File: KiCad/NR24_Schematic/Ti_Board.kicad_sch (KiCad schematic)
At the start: 23 parts, among them J5 J1 Pin J3 Pin, J5 J12 (CAN Interface w/ Transce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, J5 J4 Pin J2 Pin, J5 J5 Pin J7 Pin, J5 J8 Pin J6 Pin, J5 XBEE PRO, J6 SpeakON_NL2, Q1 Q_NMOS_DGS, Q2 Q_NMOS_DGS, Q3 Q_NMOS_DGS

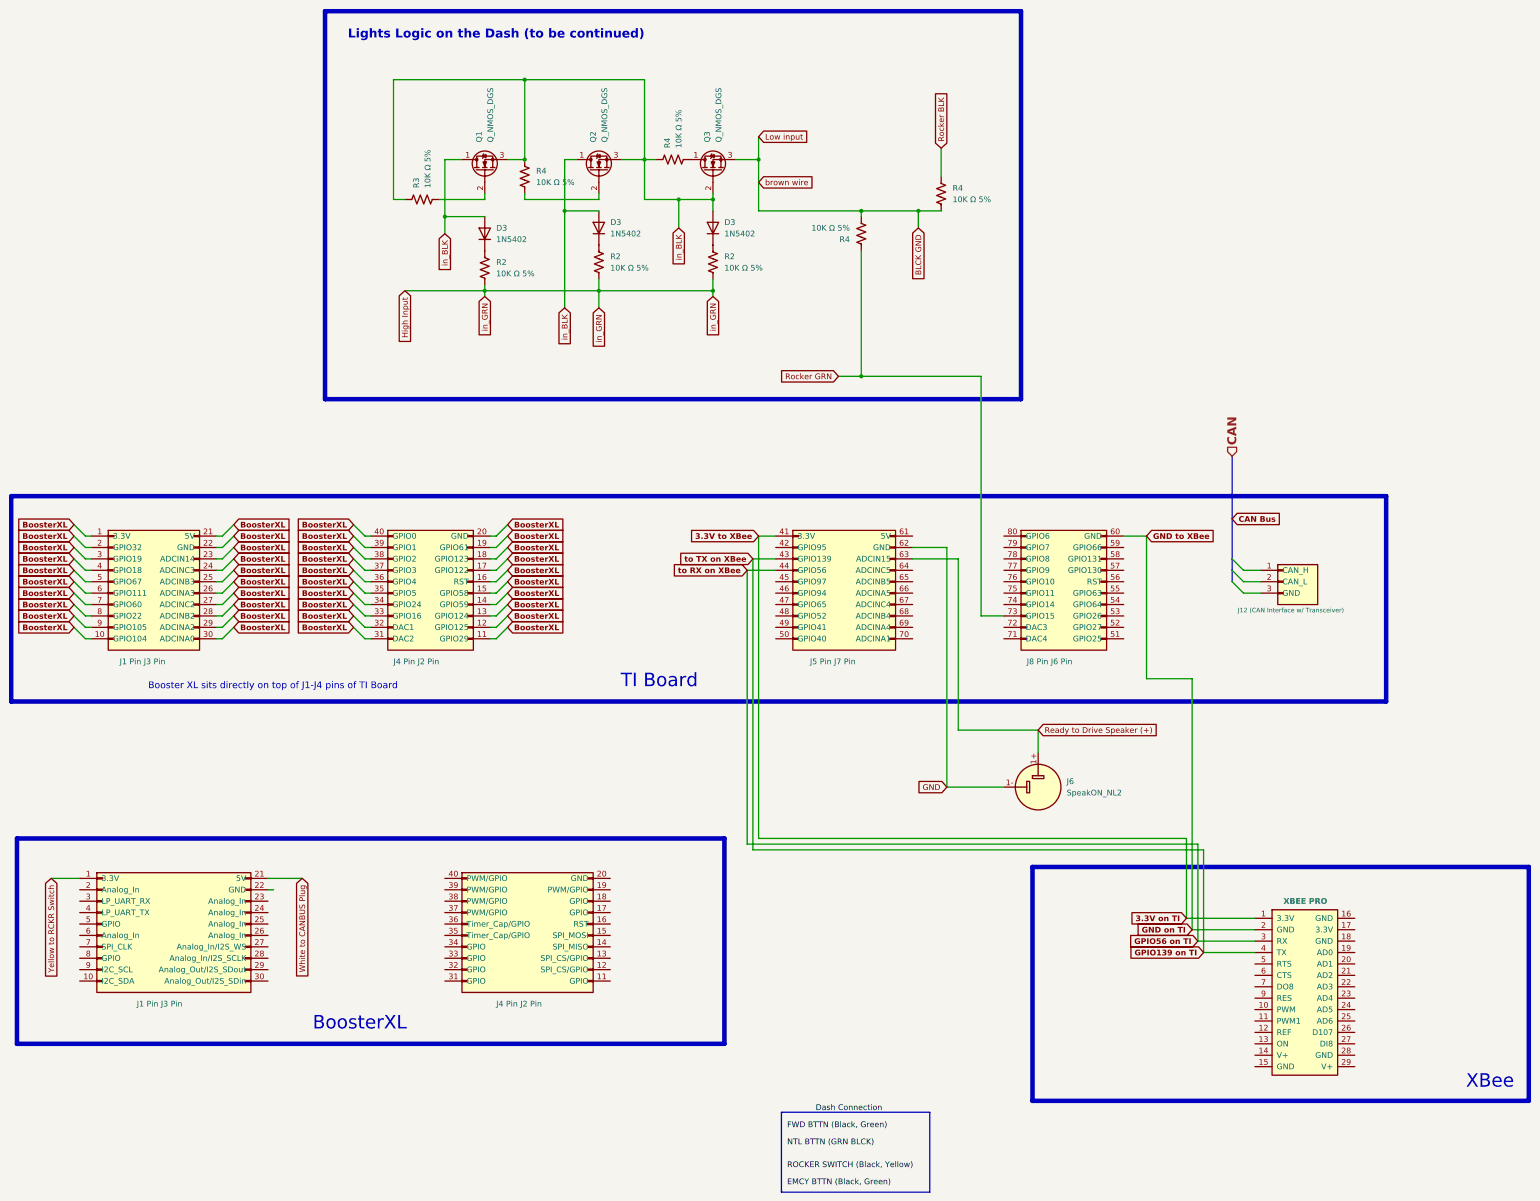
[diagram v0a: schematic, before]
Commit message: Now it is pretty :)
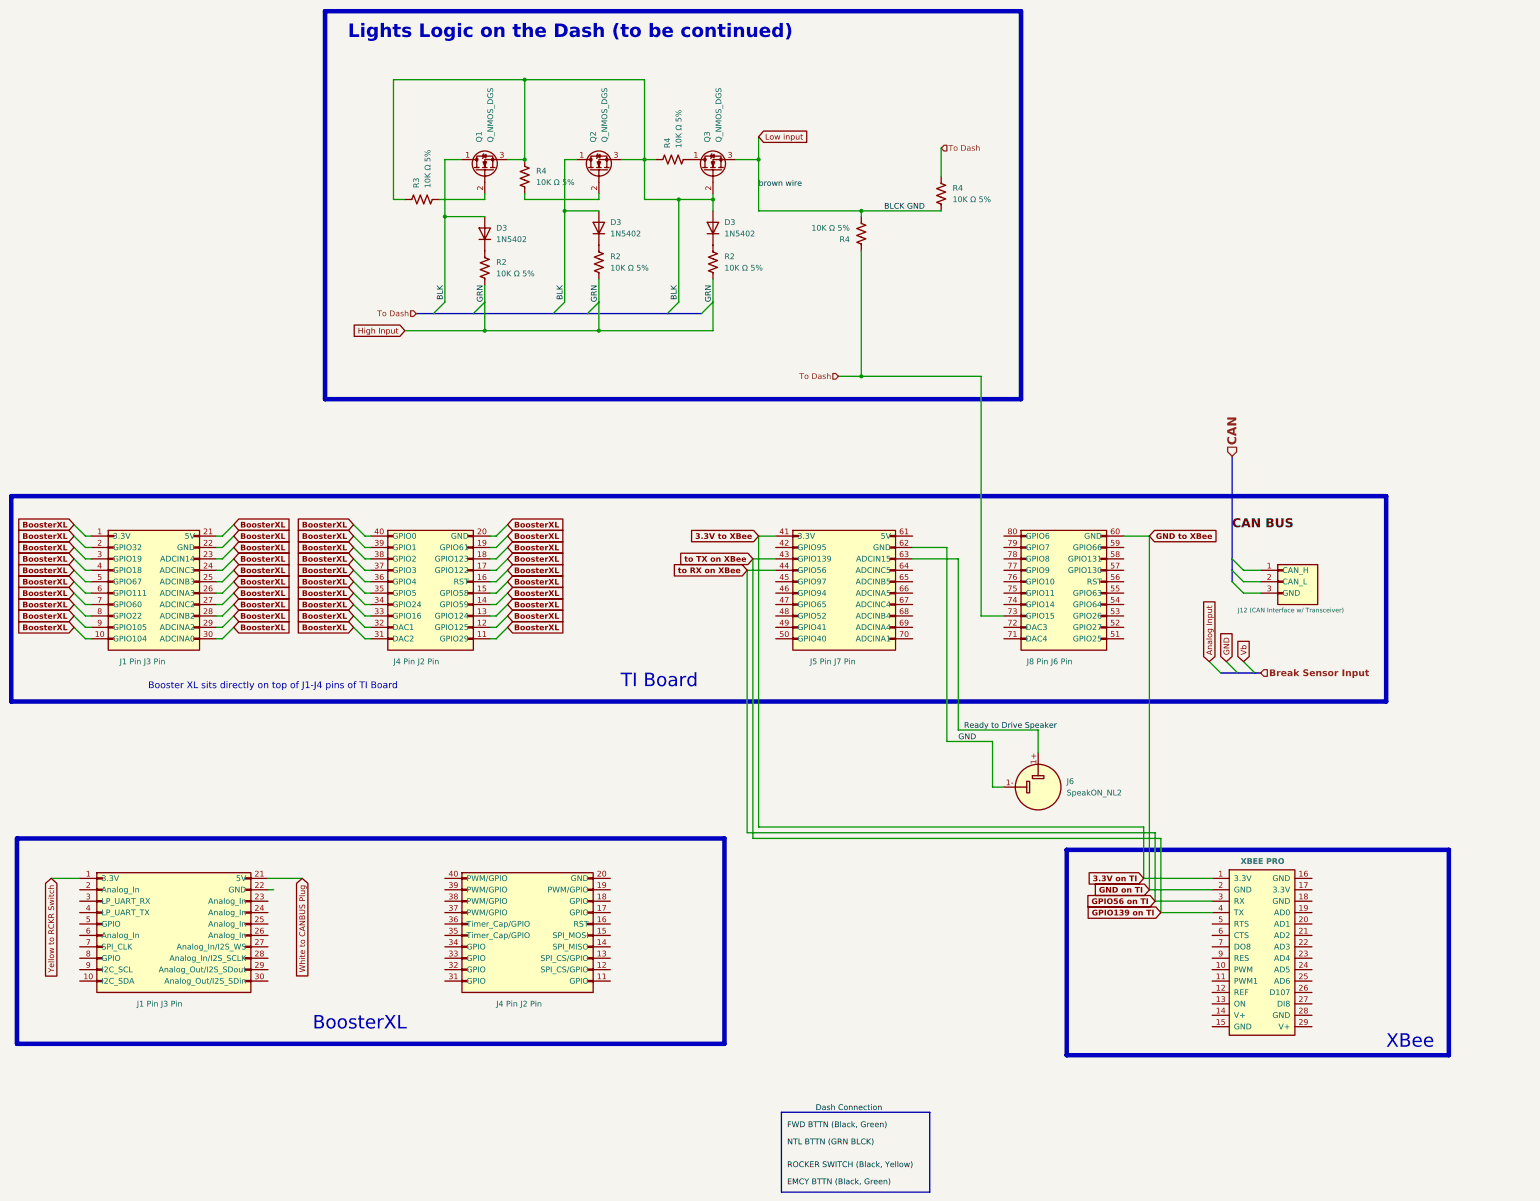
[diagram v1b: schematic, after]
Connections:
- net Rocker GRN is gone; now on net To Dash: J5.73 (GPIO15), R4.1
- net BLCK GND renamed Low input
- net Ready to Drive Speaker (+) renamed Ready to Drive Speaker
- net Rocker BLK renamed To Dash
- net in_BLK renamed BLK
